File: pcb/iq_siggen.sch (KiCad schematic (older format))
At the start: 40 parts, among them J1 Conn_Coaxial, J2 Barrel_Jack_MountingPin, J3 J3 - BANK0, U1 AMS1117-3.3, U2 TPS72325DBVR, U3 TLV73325PDBVT

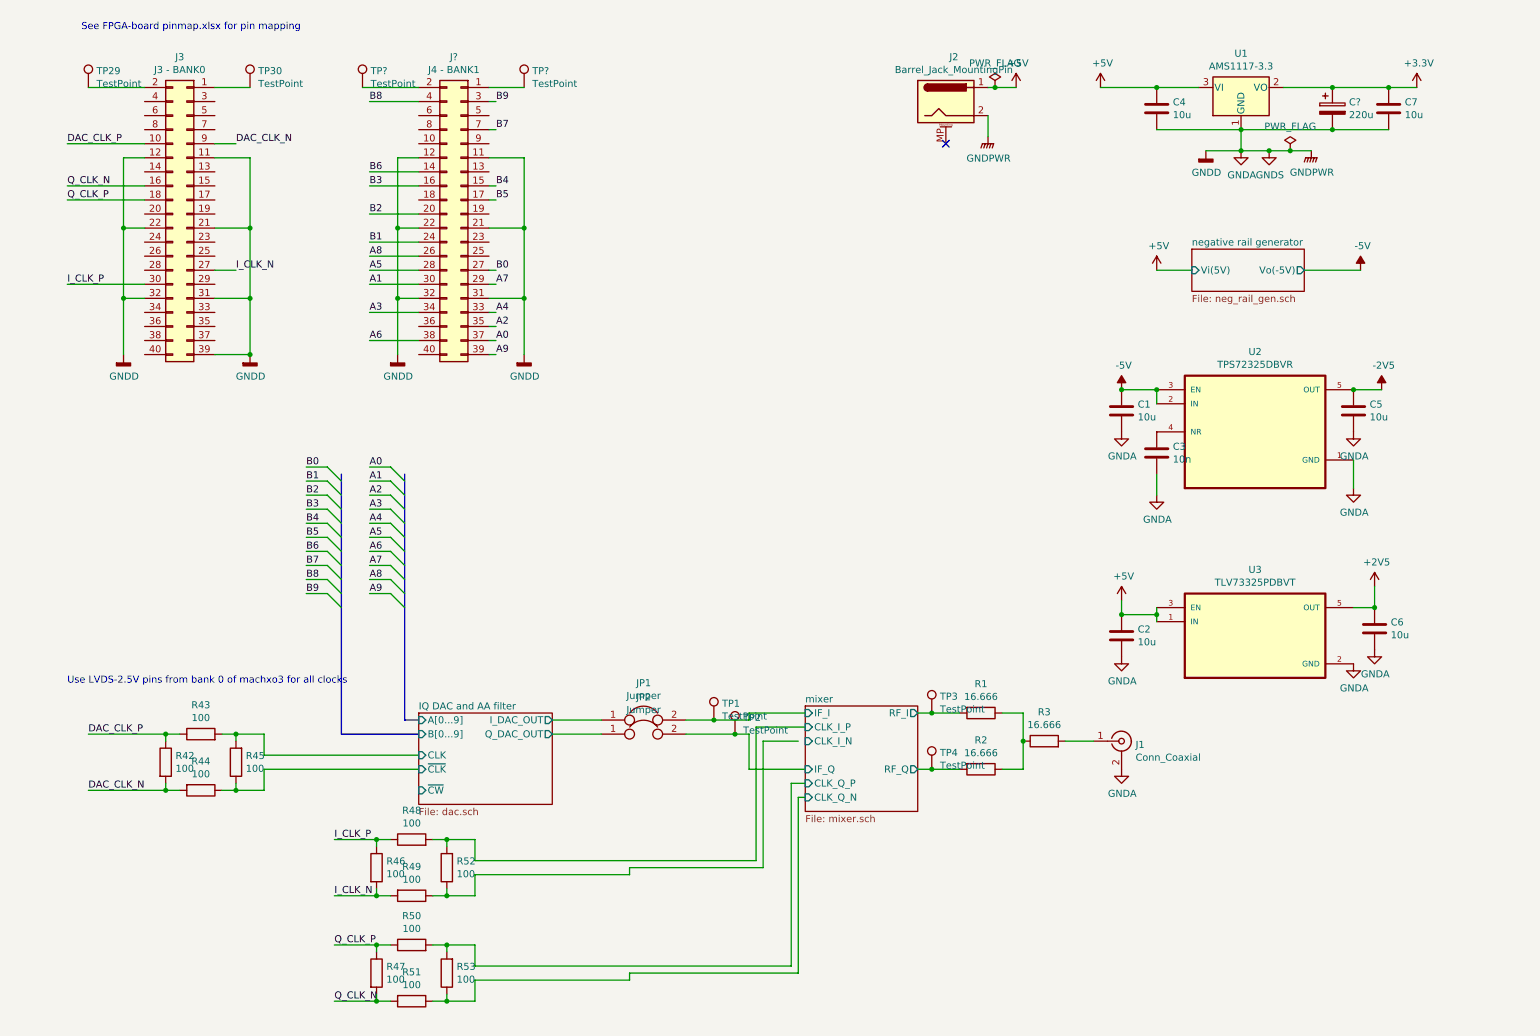
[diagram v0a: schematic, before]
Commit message: clean up ERC, more DFT stuff, started sigma delta adc
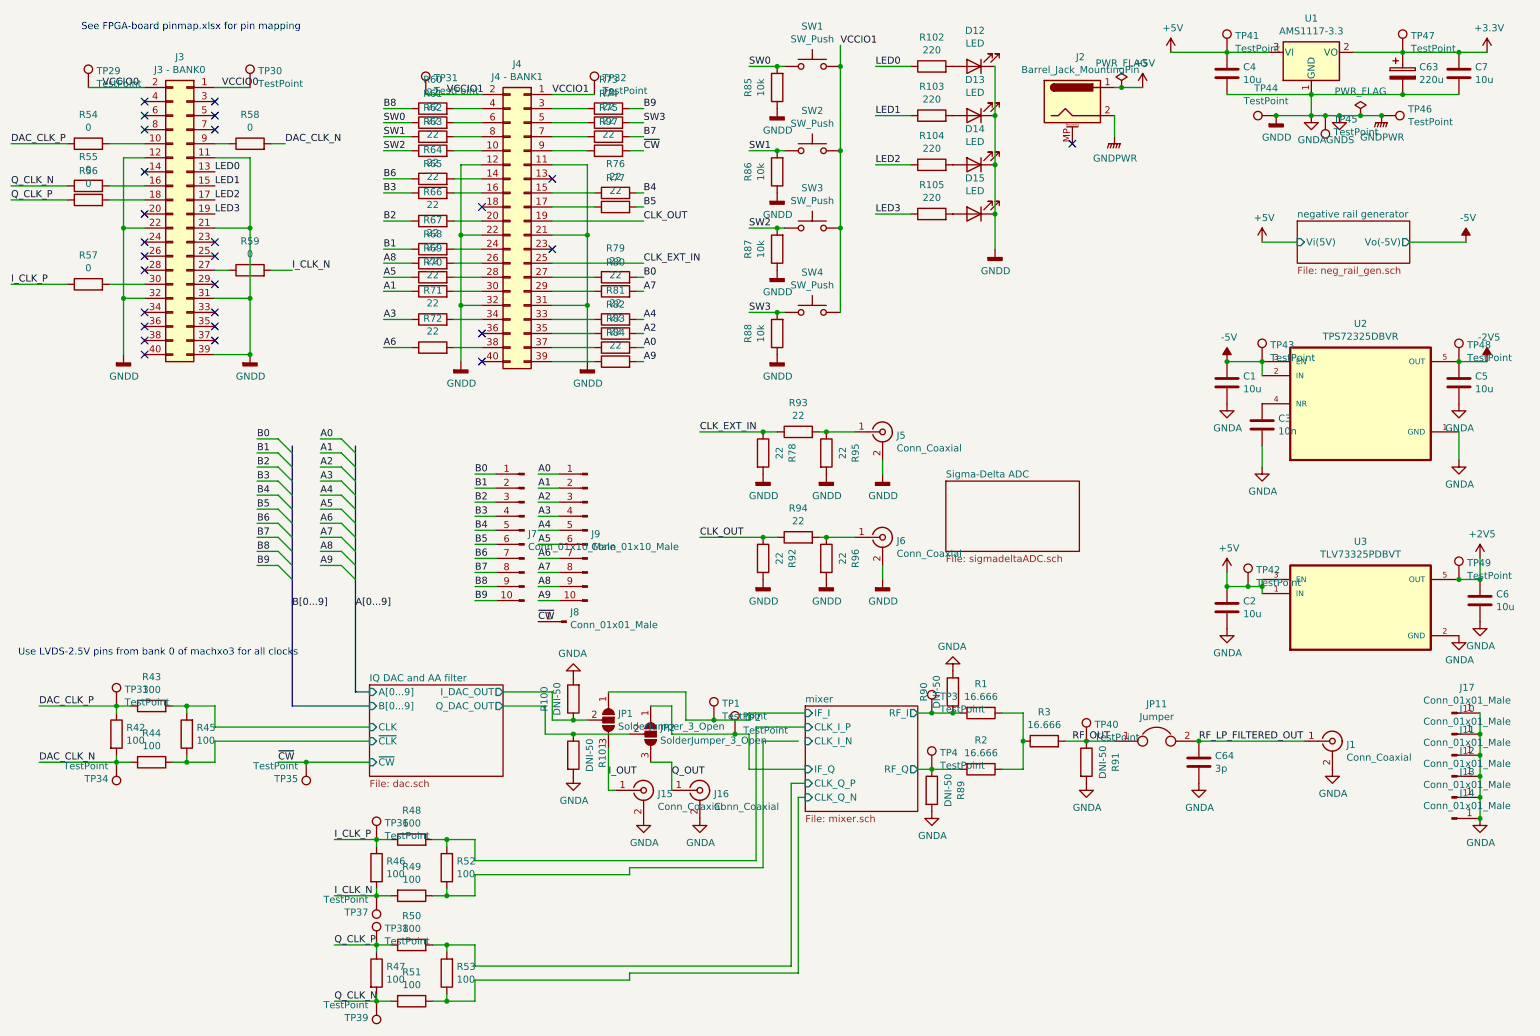
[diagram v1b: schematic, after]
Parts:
- removed JP1, JP2: Jumper, symbol Device:Jumper
- added C64: 3p, symbol Device:C
- added D12, D13, D14, D15: LED, symbol Device:LED
- added J10, J11, J12, J13, J14, J17, J8: Conn_01x01_Male, symbol Connector:Conn_01x01_Male
- added J15, J16, J5, J6: Conn_Coaxial, symbol Connector:Conn_Coaxial
- added J7, J9: Conn_01x10_Male, symbol Connector:Conn_01x10_Male
- added JP1, JP2: SolderJumper_3_Open, symbol Jumper:SolderJumper_3_Open
- added JP11: Jumper, symbol Device:Jumper
- added R100, R101, R89, R90, R91: DNI-50, symbol Device:R
- added R102, R103, R104, R105: 220, symbol Device:R
- added R54, R55, R56, R57, R58, R59: 0, symbol Device:R
- added R60, R61, R62, R63, R64, R65, R66, R67, R68, R69, R70, R71, R72, R73, R74, R75, R76, R77, R78, R79, R80, R81, R82, R83, R84, R92, R93, R94, R95, R96, R97: 22, symbol Device:R
- added R85, R86, R87, R88: 10k, symbol Device:R
- added SW1, SW2, SW3, SW4: SW_Push, symbol Switch:SW_Push
- added TP33, TP34, TP35, TP36, TP37, TP38, TP39, TP40, TP41, TP42, TP43, TP44, TP45, TP46, TP47, TP48, TP49: TestPoint, symbol Connector:TestPoint
- gave numbers to parts that had none: 4
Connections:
- net +2V5: now also TP49.1
- net +3V3: now also TP47.1
- net +5V: now also TP41.1, TP42.1
- net -2V5: now also TP48.1
- net -5V: now also TP43.1
- net A0: now also J9.1 (Pin_1), R83.2; no longer J4.37 (Pin_37)
- net A1: now also J9.2 (Pin_2), R70.1; no longer J4.30 (Pin_30)
- net A2: now also J9.3 (Pin_3), R82.2; no longer J4.35 (Pin_35)
- net A3: now also J9.4 (Pin_4), R71.1; no longer J4.34 (Pin_34)
- net A4: now also J9.5 (Pin_5), R81.2; no longer J4.33 (Pin_33)
- net A5: now also J9.6 (Pin_6), R69.1; no longer J4.28 (Pin_28)
- net A6: now also J9.7 (Pin_7), R72.1; no longer J4.38 (Pin_38)
- net A7: now also J9.8 (Pin_8), R80.2; no longer J4.29 (Pin_29)
- net A8: now also J9.9 (Pin_9), R68.1; no longer J4.26 (Pin_26)
- net A9: now also J9.10 (Pin_10), R84.2; no longer J4.39 (Pin_39)
- net B0: now also J7.1 (Pin_1), R79.2; no longer J4.27 (Pin_27)
- net B1: now also J7.2 (Pin_2), R67.1; no longer J4.24 (Pin_24)
- net B2: now also J7.3 (Pin_3), R66.1; no longer J4.20 (Pin_20)
- net B3: now also J7.4 (Pin_4), R65.1; no longer J4.16 (Pin_16)
- net B4: now also J7.5 (Pin_5), R76.2; no longer J4.15 (Pin_15)
- net B5: now also J7.6 (Pin_6), R77.2; no longer J4.17 (Pin_17)
- net B6: now also J7.7 (Pin_7), R64.1; no longer J4.14 (Pin_14)
- net B7: now also J7.8 (Pin_8), R75.2; no longer J4.7 (Pin_7)
- net B8: now also J7.9 (Pin_9), R60.1; no longer J4.4 (Pin_4)
- net B9: now also J7.10 (Pin_10), R73.2; no longer J4.3 (Pin_3)
- net DAC_CLK_N: now also R58.2, TP34.1; no longer J3.9 (Pin_9)
- net DAC_CLK_P: now also R54.1, TP33.1; no longer J3.10 (Pin_10)
- net GNDA: now also C64.2, D12.1 (K), D13.1 (K), D14.1 (K), D15.1 (K), J10.1 (Pin_1), J11.1 (Pin_1), J12.1 (Pin_1), J13.1 (Pin_1), J14.1 (Pin_1), J15.2 (Ext), J16.2 (Ext), J17.1 (Pin_1), J5.2 (Ext), J6.2 (Ext), R100.2, R101.2, R78.2, R85.1, R86.1, R87.1, R88.1, R89.2, R90.2, R91.2, R92.2, R95.2, R96.2, TP44.1, TP45.1, TP46.1
- net IQ DAC and AA filter/I_DAC_OUT: now also JP1.2 (C), R100.1
- net IQ DAC and AA filter/Q_DAC_OUT: now also JP2.2 (C), R101.1
- net I_CLK_N: now also R59.2, TP37.1; no longer J3.27 (Pin_27)
- net I_CLK_P: now also R57.1, TP36.1; no longer J3.30 (Pin_30)
- net Q_CLK_N: now also R55.1, TP39.1; no longer J3.16 (Pin_16)
- net Q_CLK_P: now also R56.1, TP38.1; no longer J3.18 (Pin_18)
- net mixer/IF_I: now also JP1.1 (A)
- net mixer/IF_Q: now also JP2.1 (A)
- net mixer/RF_I: now also R90.1
- net mixer/RF_Q: now also R89.1
- net RF_LP_FILTERED_OUT: now reaches J1.1 (In)
- net RF_LP_FILTERED_OUT: now also C64.1, JP11.2; no longer R3.2
- net VCCIO0: now reaches J3.1 (Pin_1), TP30.1
- net VCCIO0: now also J3.2 (Pin_2), TP29.1
- net LED0: now reaches J3.13 (Pin_13)
- net LED0: now also R102.1
- net LED1: now reaches J3.15 (Pin_15)
- net LED1: now also R103.1
- net LED2: now reaches J3.17 (Pin_17)
- net LED2: now also R104.1
- net LED3: now reaches J3.19 (Pin_19)
- net LED3: now also R105.1
- net VCCIO1: now reaches J4.1 (Pin_1), TP32.1
- net VCCIO1: now also J4.2 (Pin_2), TP31.1, SW1.2, SW2.2, SW3.2, SW4.2
- net at J4.10 (Pin_10): now also R63.2
- net CLK_OUT: now reaches J4.19 (Pin_19)
- net CLK_OUT: now also R92.1, R94.1
- net CLK_EXT_IN: now reaches J4.25 (Pin_25)
- net CLK_EXT_IN: now also R78.1, R93.1
- net at J4.5 (Pin_5): now also R74.1
- net at J4.6 (Pin_6): now also R61.2
- net at J4.8 (Pin_8): now also R62.2
- net at J4.9 (Pin_9): now also R97.1
- new net: J3.10 (Pin_10), R54.2
- new net: J3.16 (Pin_16), R55.2
- new net: J3.18 (Pin_18), R56.2
- new net: J3.27 (Pin_27), R59.1
- new net: J3.30 (Pin_30), R57.2
- new net: J3.9 (Pin_9), R58.1
- new net: J4.14 (Pin_14), R64.2
- new net: J4.15 (Pin_15), R76.1
- new net: J4.16 (Pin_16), R65.2
- new net: J4.17 (Pin_17), R77.1
- new net: J4.20 (Pin_20), R66.2
- new net: J4.24 (Pin_24), R67.2
- new net: J4.26 (Pin_26), R68.2
- new net: J4.27 (Pin_27), R79.1
- new net: J4.28 (Pin_28), R69.2
- new net: J4.29 (Pin_29), R80.1
- new net: J4.3 (Pin_3), R73.1
- new net: J4.30 (Pin_30), R70.2
- new net: J4.33 (Pin_33), R81.1
- new net: J4.34 (Pin_34), R71.2
- new net: J4.35 (Pin_35), R82.1
- new net: J4.37 (Pin_37), R83.1
- new net: J4.38 (Pin_38), R72.2
- new net: J4.39 (Pin_39), R84.1
- new net: J4.4 (Pin_4), R60.2
- new net: J4.7 (Pin_7), R75.1
- new net: J5.1 (In), R93.2, R95.1
- new net: J6.1 (In), R94.2, R96.1
- new net: D15.2 (A), R105.2
- new net: D12.2 (A), R102.2
- new net: D13.2 (A), R103.2
- new net: D14.2 (A), R104.2
- new net I_OUT: J15.1 (In), JP1.3 (B)
- new net Q_OUT: J16.1 (In), JP2.3 (B)
- new net RF_OUT: JP11.1, R3.2, R91.1, TP40.1
- new net SW0: R61.1, R85.2, SW1.1
- new net SW1: R62.1, R86.2, SW2.1
- new net SW2: R63.1, R87.2, SW3.1
- new net SW3: R74.2, R88.2, SW4.1
- new net ~CW: J8.1 (Pin_1), R97.2, TP35.1
- no-connect marks 1 -> 27
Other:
- moved on the sheet: C1, C2, C3, C4, C5, C6, C63, C7, J1, J2, J4, R42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
